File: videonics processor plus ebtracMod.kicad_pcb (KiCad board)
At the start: 2 copper layers, 71.1 x 114.3 mm, 18 parts, among them J11 DAT_MCU, J12 DAT0, J13 DAT_DSP, J14 + -, Q17 2N3904, U10 TXS0108EPW_MODULE, U11 TXS0108EPW_MODULE, U12 TXS0108EPW_MODULE, U13 74LS241, U14 74LS241, U9 DOIT_ESP32_DevKit_v1

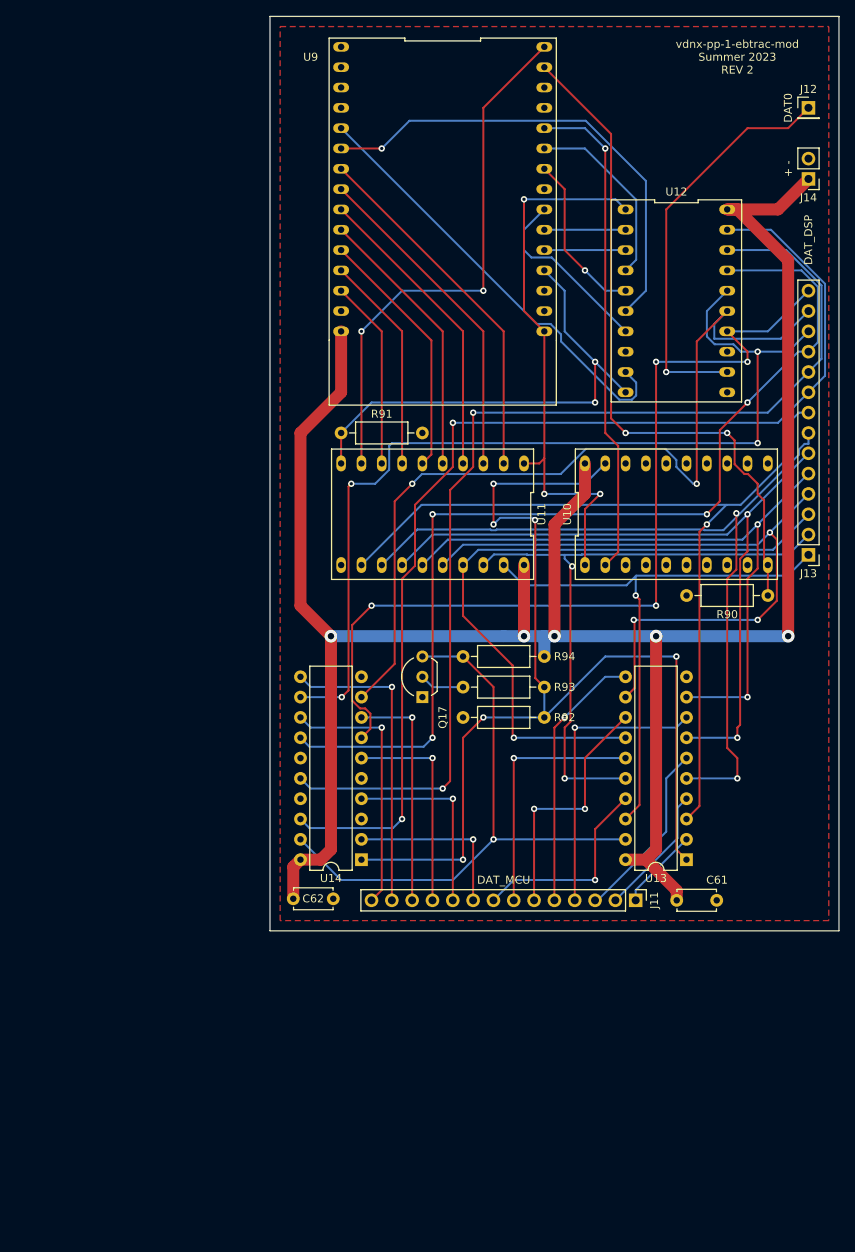
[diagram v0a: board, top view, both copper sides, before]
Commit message: PCB Redesign Finished
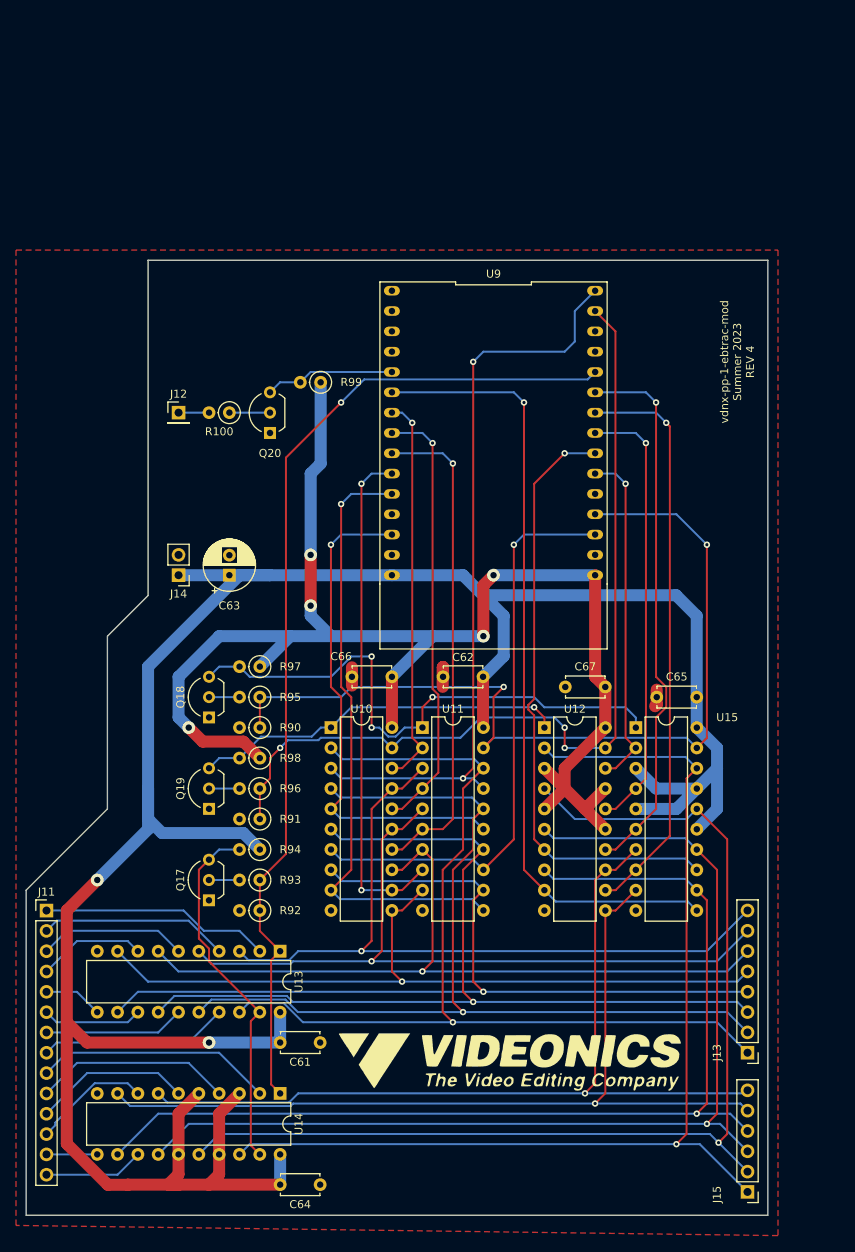
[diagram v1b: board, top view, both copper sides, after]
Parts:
- added C63: 10uF, Capacitor_THT:CP_Radial_D6.3mm_P2.50mm, F.Cu at (82.5, 105.4)
- added C64: 100nF, Capacitor_THT:C_Disc_D4.7mm_W2.5mm_P5.00mm, F.Cu at (88.9, 181.6)
- added C65: 100nF, Capacitor_THT:C_Disc_D4.7mm_W2.5mm_P5.00mm, F.Cu at (141.0, 120.7)
- added C66: 100nF, Capacitor_THT:C_Disc_D4.7mm_W2.5mm_P5.00mm, F.Cu at (102.9, 118.1)
- added C67: 100nF, Capacitor_THT:C_Disc_D4.7mm_W2.5mm_P5.00mm, F.Cu at (129.5, 119.4)
- added G***: LOGO, LOGO, F.Cu at (118.0, 166.1)
- added J15: DAT_DSP_9..14, Connector_PinHeader_2.54mm:PinHeader_1x06_P2.54mm_Vertical, F.Cu at (147.3, 182.5)
- added Q18: 2N3904, Package_TO_SOT_THT:TO-92_Inline_Wide, F.Cu at (80.0, 123.2)
- added Q19: 2N3904, Package_TO_SOT_THT:TO-92_Inline_Wide, F.Cu at (80.0, 134.6)
- added Q20: 2N3904, Package_TO_SOT_THT:TO-92_Inline_Wide, F.Cu at (87.6, 87.6)
- added R100: 220k, Resistor_THT:R_Axial_DIN0207_L6.3mm_D2.5mm_P2.54mm_Vertical, F.Cu at (82.5, 85.1)
- added R95: 1k, Resistor_THT:R_Axial_DIN0207_L6.3mm_D2.5mm_P2.54mm_Vertical, F.Cu at (86.4, 120.7)
- added R96: 1k, Resistor_THT:R_Axial_DIN0207_L6.3mm_D2.5mm_P2.54mm_Vertical, F.Cu at (86.4, 132.1)
- added R97: 10k, Resistor_THT:R_Axial_DIN0207_L6.3mm_D2.5mm_P2.54mm_Vertical, F.Cu at (86.4, 116.8)
- added R98: 10k, Resistor_THT:R_Axial_DIN0207_L6.3mm_D2.5mm_P2.54mm_Vertical, F.Cu at (86.4, 128.3)
- added R99: 10k, Resistor_THT:R_Axial_DIN0207_L6.3mm_D2.5mm_P2.54mm_Vertical, F.Cu at (94.0, 81.3)
- added U15: 74LS241, Package_DIP:DIP-20_W7.62mm, F.Cu at (133.4, 124.5)
- J13: value DAT_DSP -> DAT_DSP_1..8; footprint Connector_PinHeader_2.54mm:PinHeader_1x14_P2.54mm_Vertical -> Connector_PinHeader_2.54mm:PinHeader_1x08_P2.54mm_Vertical
- R90, R91, R92, R93, R94: footprint Resistor_THT:R_Axial_DIN0207_L6.3mm_D2.5mm_P10.16mm_Horizontal -> Resistor_THT:R_Axial_DIN0207_L6.3mm_D2.5mm_P2.54mm_Vertical
- U10, U11, U12: value TXS0108EPW_MODULE -> 74LS241; footprint videonics processor plus - Copy:DIP-20_500_ELL -> Package_DIP:DIP-20_W7.62mm
- moved J14 93.0 mm to (76.2, 105.4)
- moved J12 87.5 mm to (76.2, 85.1)
- moved J11 73.7 mm to (59.7, 147.3), turned to 0 degrees
- moved R90 65.6 mm to (86.4, 124.5)
- moved J13 62.7 mm to (147.3, 165.1)
- moved U12 55.8 mm to (121.9, 124.5), turned to 0 degrees
- moved C61 52.7 mm to (88.9, 163.8)
- moved U13 52.1 mm to (88.9, 152.4), turned to -90 degrees
- moved U10 50.7 mm to (95.3, 124.5)
- moved R91 49.3 mm to (86.4, 135.9), turned to 180 degrees
- moved R92 43.0 mm to (86.4, 147.3)
- moved R94 43.0 mm to (86.4, 139.7)
- moved R93 43.0 mm to (86.4, 143.5)
- moved Q17 36.8 mm to (80.0, 146.1)
- moved C62 36.5 mm to (114.3, 118.1), turned to 180 degrees
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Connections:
- R90 pad 1: /ESP32/BUF_CTL_LEVEL_SHIFTER_OE -> /ESP32/HIJACK
- R91 pad 1: /ESP32/DAT_BUS_LEVEL_SHIFTER_OE -> /ESP32/LISTEN
- R92 pad 1: /DAT Bus Buffer/~{DAT_BUF_OE} -> /ESP32/~{BUF_OE}
- R93 pad 1: /DAT Bus Buffer/~{DAT_BUF_OE} -> /ESP32/~{BUF_OE}
- U10 pad 1: +3.3V -> Net-(Q19-Pad3)
- U10 pad 10: /ESP32/BUF_CTL_LEVEL_SHIFTER_OE -> GND
- U10 pad 11: GND -> /DAT Bus Buffer/DAT_DSP5
- U10 pad 12: unconnected-(U10-Pad12) -> /ESP32/DAT_ESP4
- U10 pad 13: unconnected-(U10-Pad13) -> /DAT Bus Buffer/DAT_DSP6
- U10 pad 14: unconnected-(U10-Pad14) -> /ESP32/DAT_ESP3
- U10 pad 15: unconnected-(U10-Pad15) -> /DAT Bus Buffer/DAT_DSP7
- U10 pad 16: unconnected-(U10-Pad16) -> /ESP32/DAT_ESP2
- U10 pad 17: unconnected-(U10-Pad17) -> /DAT Bus Buffer/DAT_DSP8
- U10 pad 18: unconnected-(U10-Pad18) -> /ESP32/DAT_ESP1
- U10 pad 19: /DAT Bus Buffer/~{DAT_BUF_OE} -> /ESP32/LISTEN
- U10 pad 2: /ESP32/~{BUF_OE} -> /DAT Bus Buffer/DAT_DSP1
- U10 pad 20: +5V -> +3.3V
- U10 pad 3: unconnected-(U10-Pad3) -> /ESP32/DAT_ESP8
- U10 pad 4: unconnected-(U10-Pad4) -> /DAT Bus Buffer/DAT_DSP2
- U10 pad 5: unconnected-(U10-Pad5) -> /ESP32/DAT_ESP7
- U10 pad 6: unconnected-(U10-Pad6) -> /DAT Bus Buffer/DAT_DSP3
- U10 pad 7: unconnected-(U10-Pad7) -> /ESP32/DAT_ESP6
- U10 pad 8: unconnected-(U10-Pad8) -> /DAT Bus Buffer/DAT_DSP4
- U10 pad 9: unconnected-(U10-Pad9) -> /ESP32/DAT_ESP5
- U11 pad 1: +3.3V -> Net-(Q18-Pad3)
- U11 pad 10: /ESP32/DAT_BUS_LEVEL_SHIFTER_OE -> GND
- U11 pad 11: GND -> /ESP32/DAT_ESP5
- U11 pad 12: /DAT Bus Buffer/DAT_DSP8 -> /DAT Bus Buffer/DAT_DSP4
- U11 pad 13: /DAT Bus Buffer/DAT_DSP7 -> /ESP32/DAT_ESP6
- U11 pad 14: /DAT Bus Buffer/DAT_DSP6 -> /DAT Bus Buffer/DAT_DSP3
- U11 pad 15: /DAT Bus Buffer/DAT_DSP5 -> /ESP32/DAT_ESP7
- U11 pad 16: /DAT Bus Buffer/DAT_DSP4 -> /DAT Bus Buffer/DAT_DSP2
- U11 pad 17: /DAT Bus Buffer/DAT_DSP3 -> /ESP32/DAT_ESP8
- U11 pad 18: /DAT Bus Buffer/DAT_DSP2 -> /DAT Bus Buffer/DAT_DSP1
- U11 pad 19: /DAT Bus Buffer/DAT_DSP1 -> /ESP32/HIJACK
- U11 pad 3: /ESP32/DAT_ESP2 -> /DAT Bus Buffer/DAT_DSP8
- U11 pad 4: /ESP32/DAT_ESP3 -> /ESP32/DAT_ESP2
- U11 pad 5: /ESP32/DAT_ESP4 -> /DAT Bus Buffer/DAT_DSP7
- U11 pad 6: /ESP32/DAT_ESP5 -> /ESP32/DAT_ESP3
- U11 pad 7: /ESP32/DAT_ESP6 -> /DAT Bus Buffer/DAT_DSP6
- U11 pad 8: /ESP32/DAT_ESP7 -> /ESP32/DAT_ESP4
- U11 pad 9: /ESP32/DAT_ESP8 -> /DAT Bus Buffer/DAT_DSP5
- U12 pad 1: +3.3V -> Net-(Q19-Pad3)
- U12 pad 10: /ESP32/DAT_BUS_LEVEL_SHIFTER_OE -> GND
- U12 pad 11: GND -> /DAT Bus Buffer/DAT_DSP13
- U12 pad 12: /Device Settings Processor/DAT_DSP0 -> /ESP32/DAT_ESP12
- U12 pad 13: unconnected-(U12-Pad13) -> /DAT Bus Buffer/DAT_DSP14
- U12 pad 14: /DAT Bus Buffer/DAT_DSP14 -> /ESP32/DAT_ESP11
- U12 pad 15: /DAT Bus Buffer/DAT_DSP13 -> +3.3V
- U12 pad 16: /DAT Bus Buffer/DAT_DSP12 -> /ESP32/DAT_ESP10
- U12 pad 17: /DAT Bus Buffer/DAT_DSP11 -> +3.3V
- U12 pad 18: /DAT Bus Buffer/DAT_DSP10 -> /ESP32/DAT_ESP9
- U12 pad 19: /DAT Bus Buffer/DAT_DSP9 -> /ESP32/LISTEN
- U12 pad 2: /ESP32/DAT_ESP9 -> /DAT Bus Buffer/DAT_DSP9
- U12 pad 20: +5V -> +3.3V
- U12 pad 3: /ESP32/DAT_ESP10 -> +3.3V
- U12 pad 4: /ESP32/DAT_ESP11 -> /DAT Bus Buffer/DAT_DSP10
- U12 pad 5: /ESP32/DAT_ESP12 -> +3.3V
- U12 pad 6: /ESP32/DAT_ESP13 -> /DAT Bus Buffer/DAT_DSP11
- U12 pad 8: unconnected-(U12-Pad8) -> /DAT Bus Buffer/DAT_DSP12
- U12 pad 9: /ESP32/DAT_ESP0 -> /ESP32/DAT_ESP13
- U13 pad 1: /DAT Bus Buffer/~{DAT_BUF_OE} -> /ESP32/~{BUF_OE}
- U14 pad 1: /DAT Bus Buffer/~{DAT_BUF_OE} -> /ESP32/~{BUF_OE}
- U14 pad 15: unconnected-(U14-Pad15) -> +5V
- U14 pad 17: unconnected-(U14-Pad17) -> +5V
- U14 pad 3: unconnected-(U14-Pad3) -> +5V
- U14 pad 5: unconnected-(U14-Pad5) -> +5V
- U9 pad 12: /ESP32/DAT_ESP6 -> unconnected-(U9-Pad12)
- U9 pad 18: unconnected-(U9-Pad18) -> /ESP32/DAT_ESP6
- U9 pad 19: /ESP32/DAT_BUS_LEVEL_SHIFTER_OE -> /ESP32/HIJACK
- U9 pad 20: /ESP32/DAT_ESP10 -> unconnected-(U9-Pad20)
- U9 pad 23: unconnected-(U9-Pad23) -> /ESP32/DAT_ESP10
- U9 pad 29: /ESP32/BUF_CTL_LEVEL_SHIFTER_OE -> /ESP32/LISTEN
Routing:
- net /DAT Bus Buffer/~{DAT_BUF_OE}: track 135.6 -> 0.00 mm, vias 6 -> 0
- net /ESP32/HIJACK: track 0.00 -> 112.7 mm, vias 0 -> 2
- net /ESP32/LISTEN: track 0.00 -> 112.5 mm, vias 0 -> 3
- net +3.3V: track 70.6 -> 177.9 mm, vias 3 -> 5
- net /ESP32/BUF_CTL_LEVEL_SHIFTER_OE: track 85.3 -> 0.00 mm, vias 2 -> 0
- net Net-(Q18-Pad3): track 0.00 -> 70.7 mm, vias 0 -> 3
- net /ESP32/~{BUF_OE}: track 62.1 -> 125.9 mm
- net /ESP32/DAT_BUS_LEVEL_SHIFTER_OE: track 61.7 -> 0.00 mm, vias 2 -> 0
- net +5V: track 276.5 -> 329.8 mm, vias 5 -> 2
- net /ESP32/DAT_ESP14: track 23.0 -> 76.2 mm, vias 0 -> 1
- net /ESP32/DAT_ESP12: track 20.9 -> 72.1 mm
- net /DAT Bus Buffer/DAT_DSP1: track 72.0 -> 121.0 mm
- net /Device Settings Processor/DAT_DSP0: track 51.0 -> 3.81 mm, vias 1 -> 0
- net Net-(Q19-Pad3): track 0.00 -> 46.9 mm, vias 0 -> 1
- net /ESP32/DAT_ESP6: track 27.3 -> 73.0 mm, vias 0 -> 1
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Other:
- board size 71.1 x 114.3 mm -> 92.7 x 119.4 mm
- board text added: "vdnx-pp-1-ebtrac-mod Summer 2023 REV 4"
- board text removed: "vdnx-pp-1-ebtrac-mod Summer 2023 REV 2"
